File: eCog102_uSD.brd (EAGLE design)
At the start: 48 x 28 mm, 6 parts

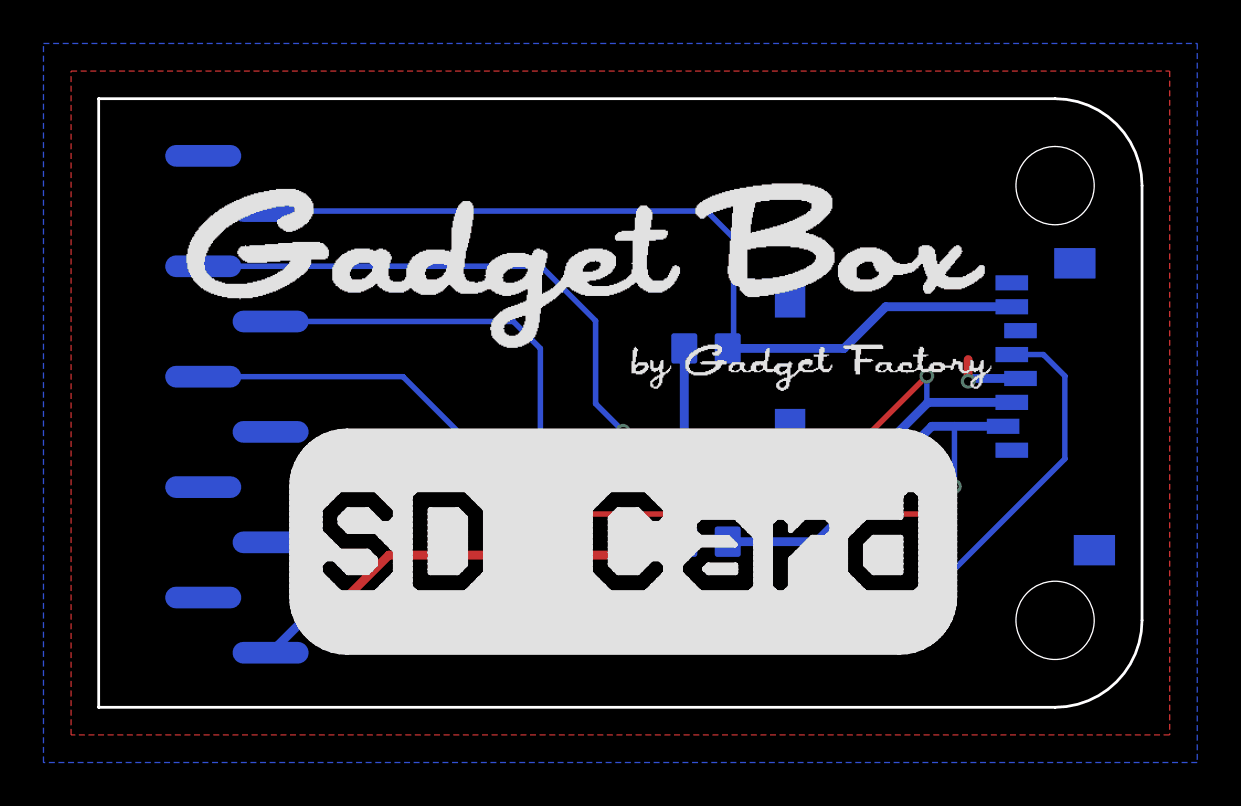
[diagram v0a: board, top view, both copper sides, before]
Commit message: Update all of the Fonts and graphics
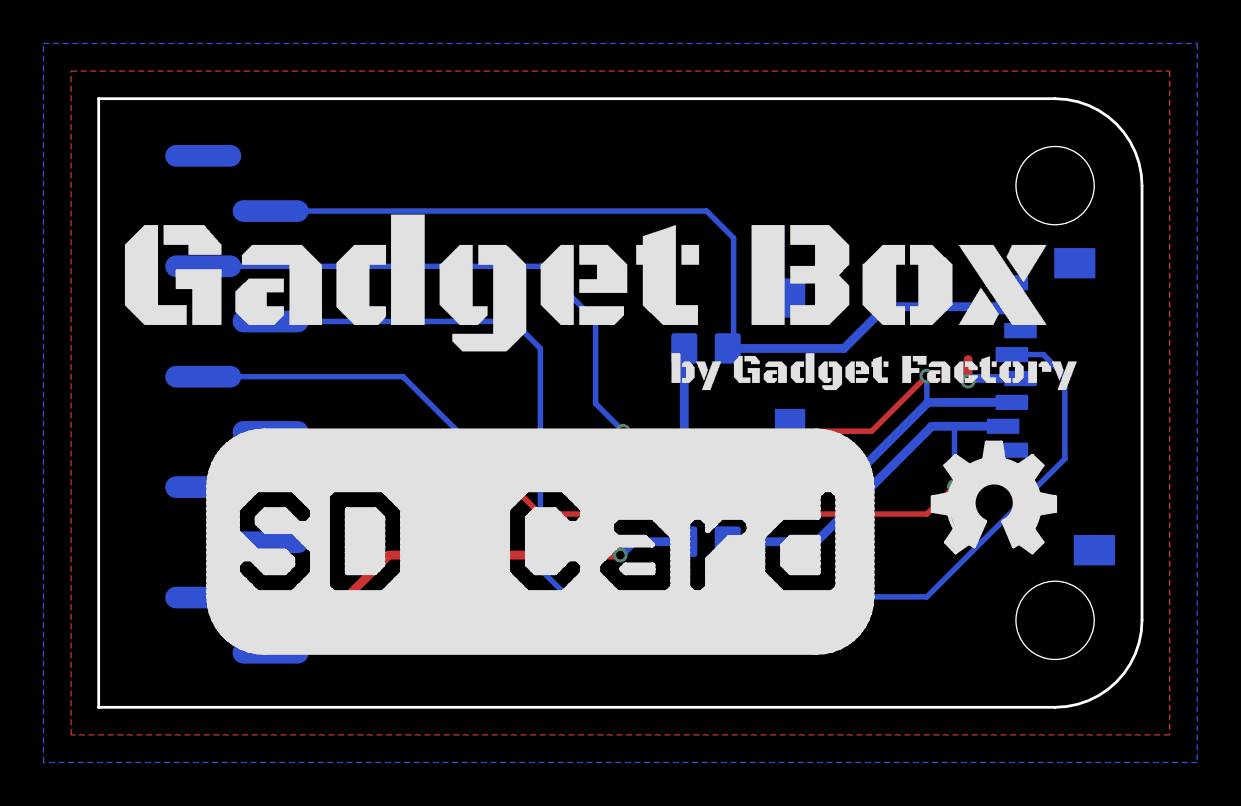
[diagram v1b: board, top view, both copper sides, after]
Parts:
- added U$2: (no value), ohw-logo:OSHW_FILLX200_NOTEXT
- moved U$1 1.09 mm to (22.5, 19.3)

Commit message: All the 2.0 updates
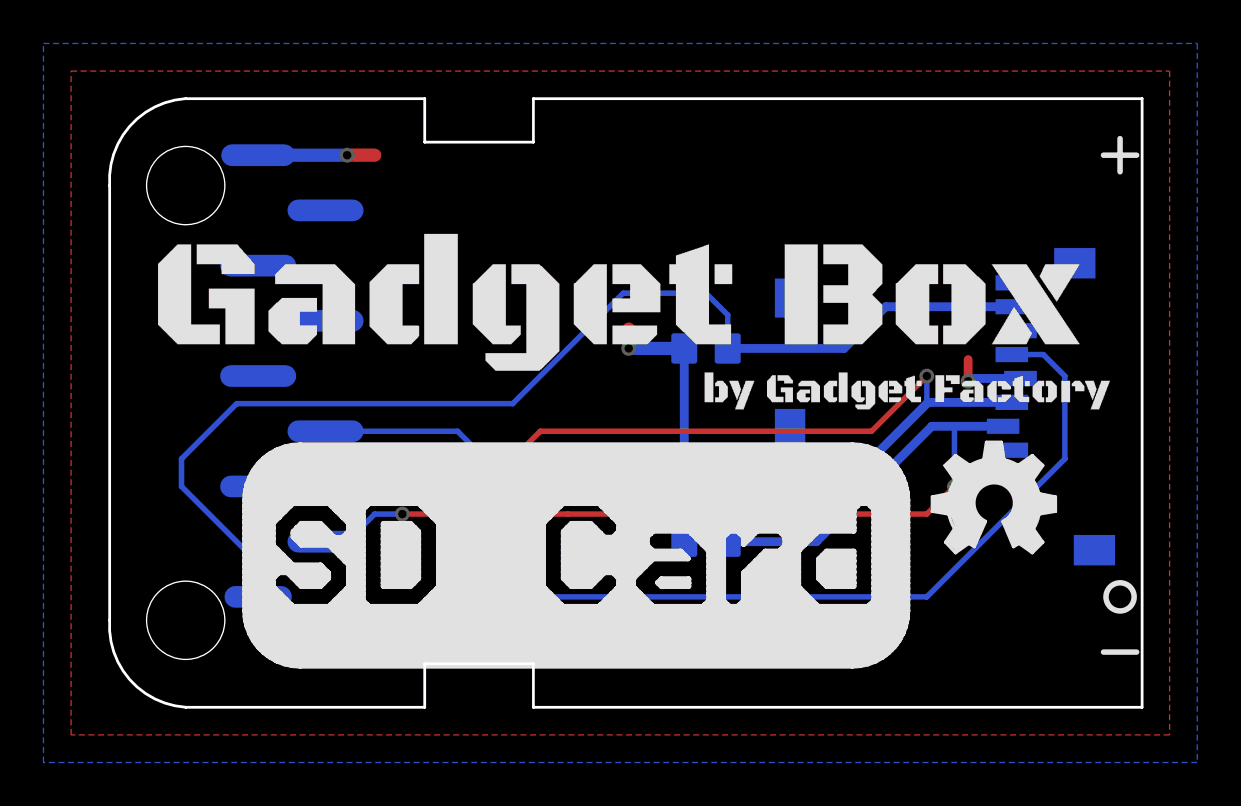
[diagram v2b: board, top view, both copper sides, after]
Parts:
- moved U$1 1.76 mm to (24.0, 18.4)
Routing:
- net 3V3: track 33.5 -> 21.2 mm
- net SD_MISO: track 40.9 -> 52.3 mm
- net SD_MOSI: track 55.7 -> 46.8 mm
- net SD_SCK: track 57.0 -> 48.5 mm
- net SD_!CS: track 55.3 -> 48.7 mm
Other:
- board size 48 x 28 mm -> 47.5 x 28 mm
- board text added: "SPI-CS"
- board text added: "SPI-MISO"
- board text added: "SPI-MOSI"
- board text added: "SPI-SCK"
- board text added: "ecog102 v2.0"
- board text removed: "SPI-CS>"
- board text removed: "SPI-MISO>"
- board text removed: "SPI-MOSI<"
- board text removed: "SPI-SCK>"
- board text removed: "ecog102 v1.1"
